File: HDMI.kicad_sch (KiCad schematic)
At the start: 10 parts, among them IC6 TPS2553QDBVRQ1, J9 HDMI_E

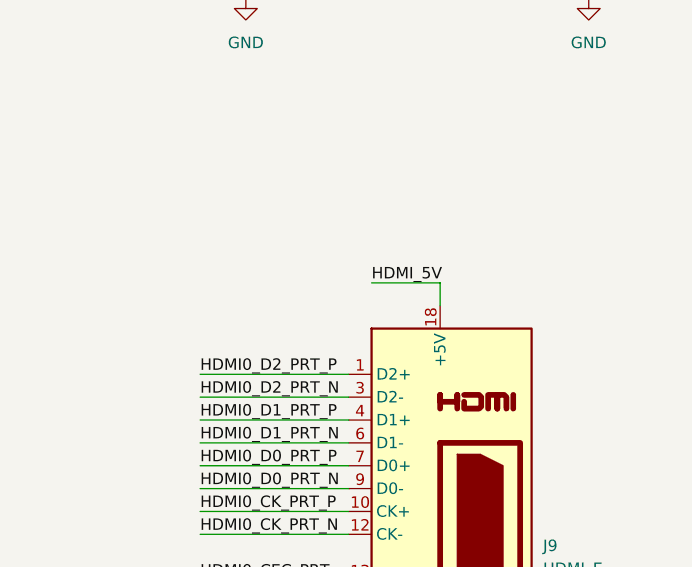
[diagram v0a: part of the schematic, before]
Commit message: changed a bunch of stuff, still have work
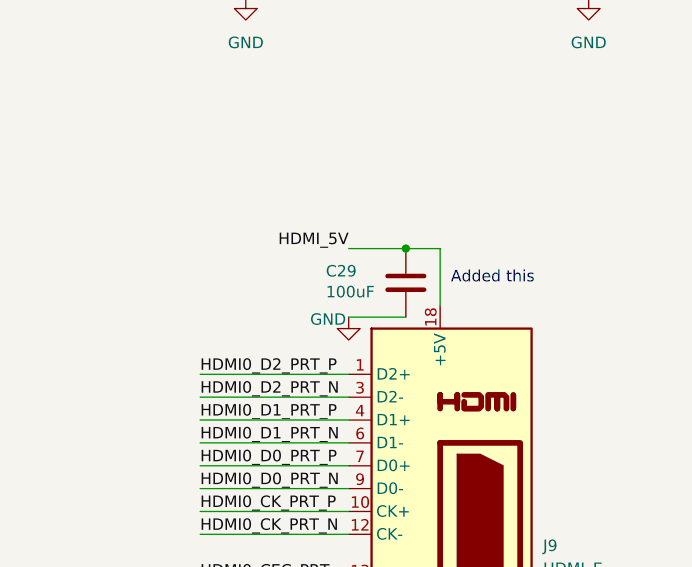
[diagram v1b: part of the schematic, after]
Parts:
- added C29: 100uF, Capacitor_SMD:C_0805_2012Metric, symbol Device:C
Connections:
- net GND: now also C29.2
- net HDMI_5V: now also C29.1
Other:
- note added: "Added this"
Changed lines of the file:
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@@
+		)
+	)
+	(text "Added this"
+		(exclude_from_sim no)
+		(at 256.032 94.742 0)
+		(effects
+			(font
+				(size 1.27 1.27)
+			)
 		)
 	)
@@
 	)
 	(junction
+		(at 246.38 91.44)
+		(diameter 0)
+		(color 0 0 0 0)
+	)
+	(junction
 		(at 34.29 69.85)
 		(diameter 1.016)
@@
 	(wire
 		(pts
+			(xy 240.03 91.44) (xy 246.38 91.44)
+		)
+		(stroke
+			(width 0)
+			(type default)
+		)
+	)
+	(wire
+		(pts
 			(xy 97.79 105.41) (xy 116.84 105.41)
 		)
@@
 	(wire
 		(pts
-			(xy 250.19 95.25) (xy 250.19 97.79)
+			(xy 250.19 91.44) (xy 250.19 97.79)
 		)
 		(stroke
@@
 	(wire
 		(pts
-			(xy 250.19 95.25) (xy 242.57 95.25)
-		)
-		(stroke
-			(width 0)
-			(type default)
-		)
-	)
-	(wire
-		(pts
 			(xy 144.78 148.59) (xy 161.29 148.59)
 		)
@@
 	(wire
 		(pts
+			(xy 240.03 99.06) (xy 246.38 99.06)
+		)
+		(stroke
+			(width 0)
+			(type default)
+		)
+	)
+	(wire
+		(pts
 			(xy 34.29 138.43) (xy 34.29 146.05)
 		)
@@
 			(width 0)
 			(type solid)
+		)
+	)
+	(wire
+		(pts
+			(xy 246.38 91.44) (xy 250.19 91.44)
+		)
+		(stroke
+			(width 0)
+			(type default)
 		)
 	)
@@
 	)
 	(label "HDMI_5V"
-		(at 242.57 95.25 0)
-		(effects
-			(font
-				(size 1.27 1.27)
-			)
-			(justify left bottom)
+		(at 240.03 91.44 180)
+		(effects
+			(font
+				(size 1.27 1.27)
+			)
+			(justify right bottom)
 		)
 	)
@@
 			)
 			(justify left)
+		)
+	)
+	(symbol
+		(lib_id "power:GND")
+		(at 240.03 99.06 0)
+		(unit 1)
+		(exclude_from_sim no)
+		(in_bom yes)
+		(on_board yes)
+		(dnp no)
+		(property "Reference" "#PWR041"
+			(at 240.03 105.41 0)
+			(effects
+				(font
+					(size 1.27 1.27)
+				)
+				(hide yes)
+			)
+		)
+		(property "Value" "GND"
+			(at 237.744 99.314 0)
+			(effects
+				(font
+					(size 1.27 1.27)
+				)
+			)
+		)
+		(property "Footprint" ""
+			(at 240.03 99.06 0)
+			(effects
+				(font
+					(size 1.27 1.27)
+				)
+				(hide yes)
+			)
+		)
+		(property "Datasheet" ""
+			(at 240.03 99.06 0)
+			(effects
+				(font
+					(size 1.27 1.27)
+				)
+				(hide yes)
+			)
+		)
+		(property "Description" "Power symbol creates a global label with name \"GND\" , ground"
+			(at 240.03 99.06 0)
+			(effects
+				(font
+					(size 1.27 1.27)
+				)
+				(hide yes)
+			)
+		)
+		(pin "1"
+		)
+		(instances
+			(project "PiBoard"
+				(path "/e4d65698-b8ec-4bf6-9f2b-a5010377155a/2dec5fd6-8756-425d-9ae9-2f1c2fc4e6c1"
+					(reference "#PWR041")
+					(unit 1)
+				)
+			)
 		)
 	)
@@
 					(unit 1)
 				)
+			)
+		)
+	)
+	(symbol
+		(lib_id "Device:C")
+		(at 246.38 95.25 0)
+		(unit 1)
+		(exclude_from_sim no)
+		(in_bom yes)
+		(on_board yes)
+		(dnp no)
+		(property "Reference" "C29"
+			(at 237.49 93.9546 0)
+			(effects
+				(font
+					(size 1.27 1.27)
+				)
+				(justify left)
+			)
+		)
+		(property "Value" "100uF"
+			(at 237.49 96.266 0)
+			(effects
+				(font
+					(size 1.27 1.27)
+				)
+				(justify left)
+			)
+		)
+		(property "Footprint" "Capacitor_SMD:C_0805_2012Metric"
+			(at 247.3452 99.06 0)
+			(effects
+				(font
+					(size 1.27 1.27)
+				)
+				(hide yes)
+			)
+		)
+		(property "Datasheet" "https://content.kemet.com/datasheets/KEM_C1002_X7R_SMD.pdf"
+			(at 246.38 95.25 0)
+			(effects
+				(font
+					(size 1.27 1.27)
+				)
+				(hide yes)
+			)
+		)
+		(property "Description" "Unpolarized capacitor"
+			(at 246.38 95.25 0)
+			(effects
+				(font
+					(size 1.27 1.27)
+				)
+				(hide yes)
+			)
+		)
+		(property "P/N" "C0805C104M5RACTU"
+			(at 246.38 95.25 0)
+			(effects
+				(font
+					(size 1.27 1.27)
+				)
+				(hide yes)
+			)
+		)
+		(pin "1"
+		)
+		(pin "2"
+		)
+		(instances
+			(project "PiBoard"
+				(path "/e4d65698-b8ec-4bf6-9f2b-a5010377155a/2dec5fd6-8756-425d-9ae9-2f1c2fc4e6c1"
+					(reference "C29")
+					(unit 1)
+				)
